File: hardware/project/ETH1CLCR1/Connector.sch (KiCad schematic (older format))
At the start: 25 parts, among them J1601 C64AC, K1601 HE3621A0510, K1602 HE3621A0510, K1603 HE3621A0510, K1604 HE3621A0510, K1605 HE3621A0510, K1606 HE3621A0510, Q1601 BC847W, Q1602 BC847W, Q1603 BC847W, Q1604 BC847W, Q1605 BC847W, Q1606 BC847W

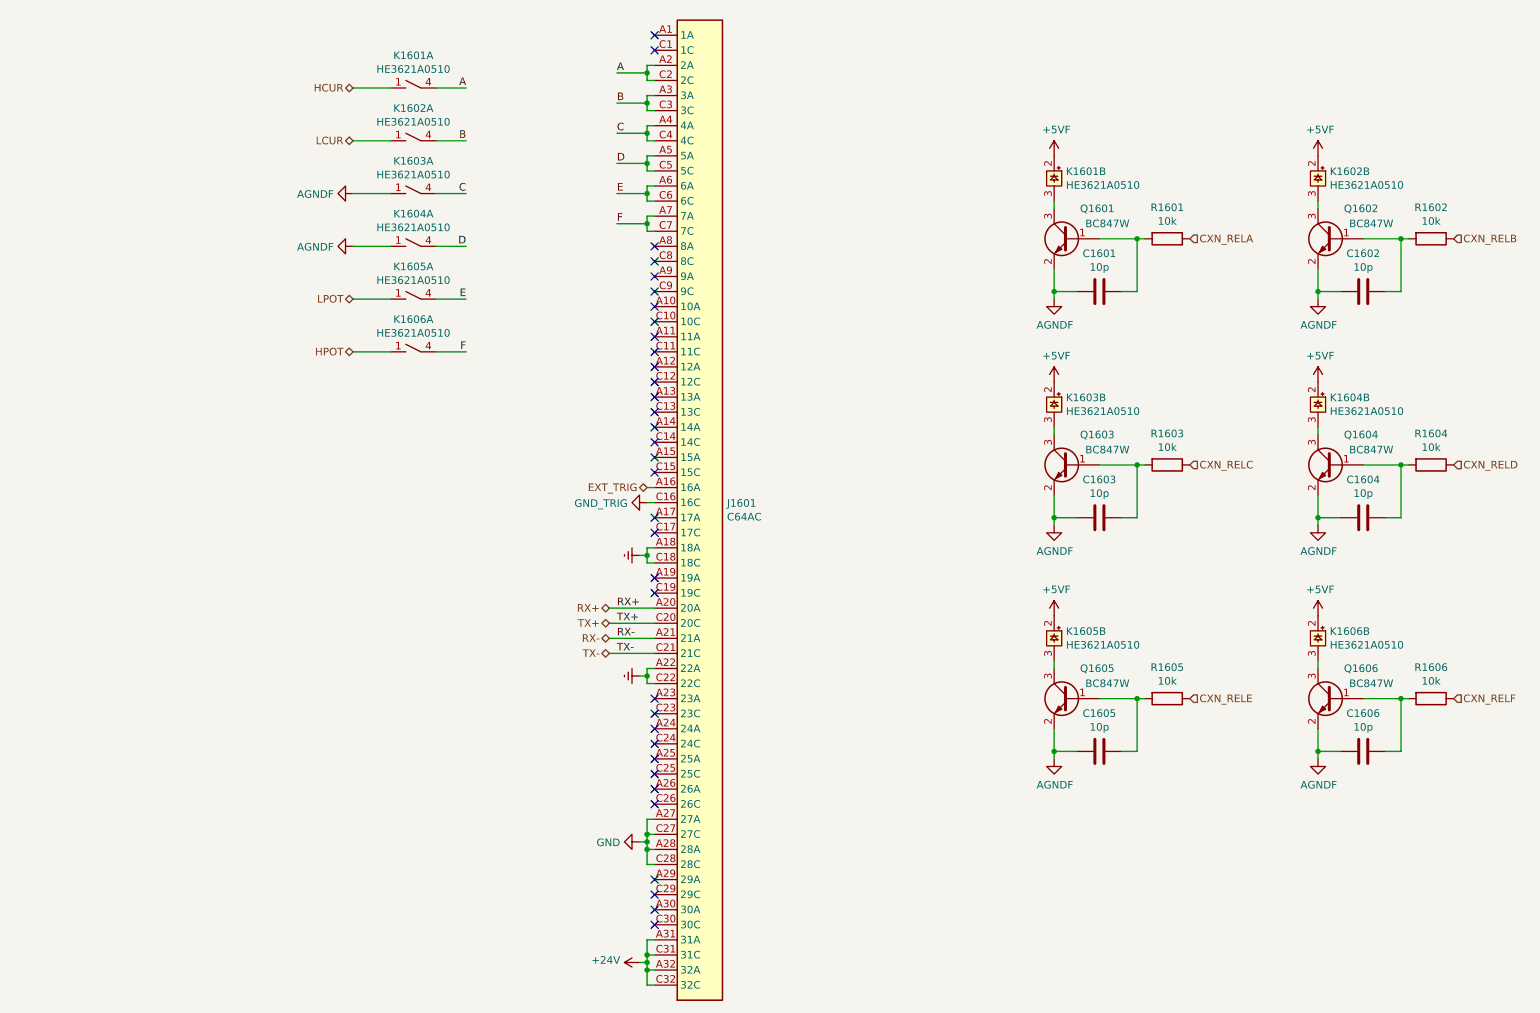
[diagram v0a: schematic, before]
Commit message: Modification in schematic and PCB layout.
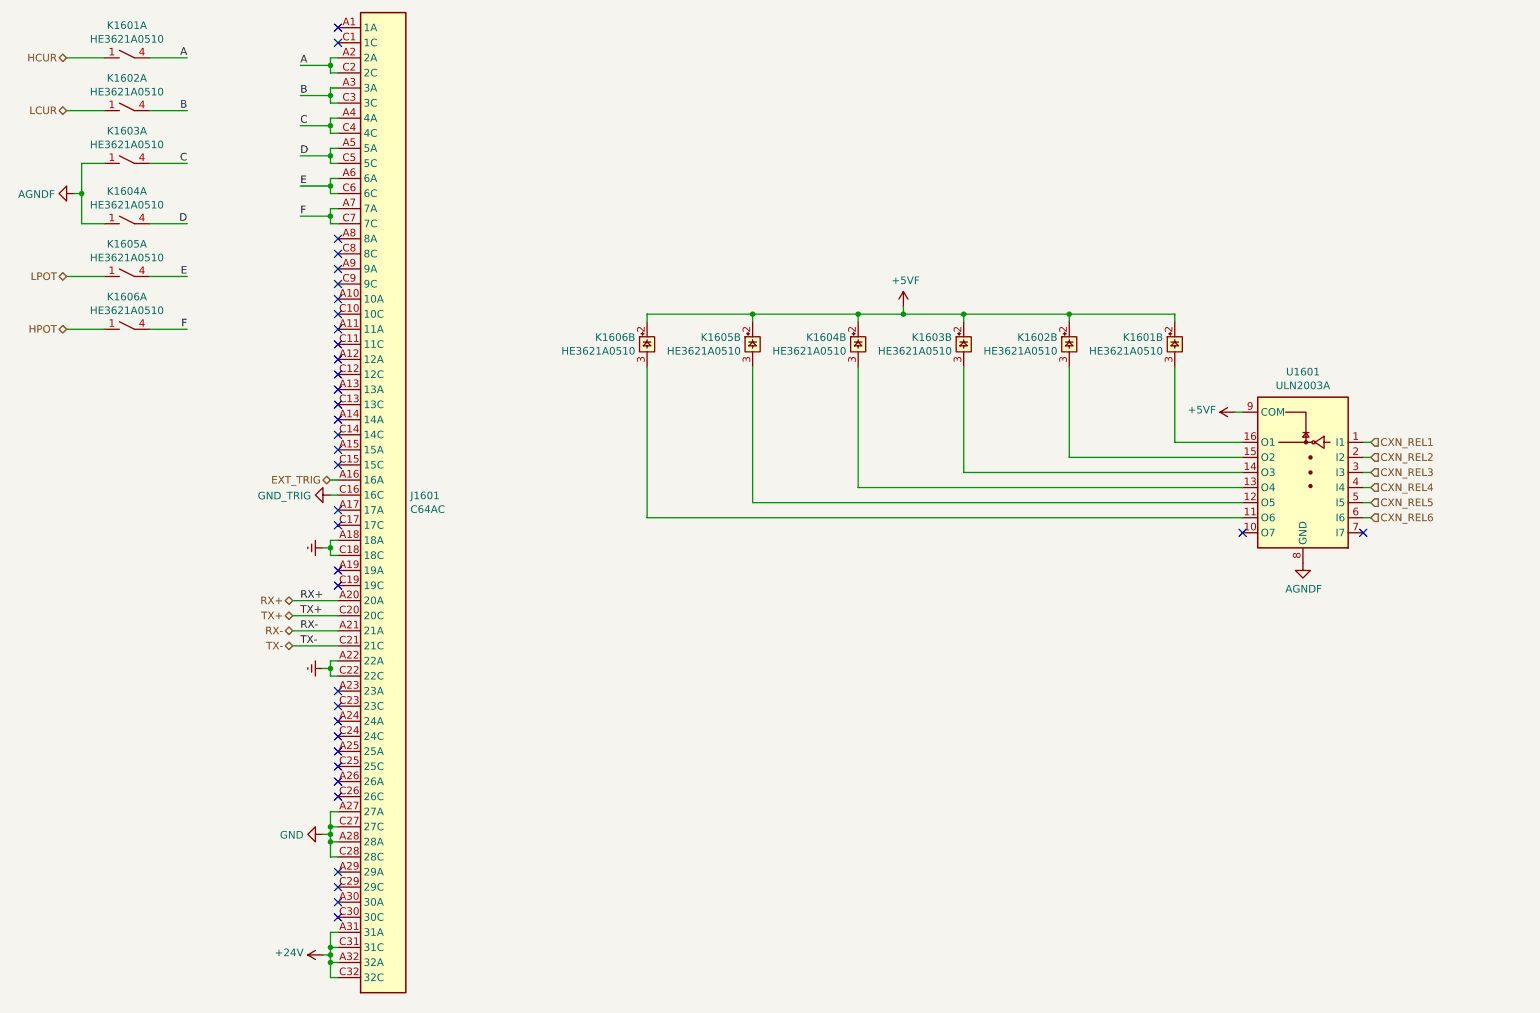
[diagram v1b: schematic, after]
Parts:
- removed C1601, C1602, C1603, C1604, C1605, C1606: 10p, Capacitor_SMD:C_0603_1608Metric_Pad1.05x0.95mm_HandSolder, symbol Device:C
- removed Q1601, Q1602, Q1603, Q1604, Q1605, Q1606: BC847W, Package_TO_SOT_SMD:SOT-323_SC-70, symbol Transistor_BJT:BC847W
- removed R1601, R1602, R1603, R1604, R1605, R1606: 10k, Resistor_SMD:R_0603_1608Metric_Pad1.05x0.95mm_HandSolder, symbol Device:R
- added U1601: ULN2003A, Package_SO:TSSOP-16_4.4x5mm_P0.65mm, symbol Transistor_Array:ULN2003A
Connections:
- net +5VF: now also U1601.9 (COM)
- net AGNDF: now also U1601.8 (GND)
- net at K1601.3: now also U1601.16 (O1)
- net at K1602.3: now also U1601.15 (O2)
- net at K1603.3: now also U1601.14 (O3)
- net at K1604.3: now also U1601.13 (O4)
- net at K1605.3: now also U1601.12 (O5)
- net at K1606.3: now also U1601.11 (O6)
- new net CXN_REL1: U1601.1 (I1)
- new net CXN_REL2: U1601.2 (I2)
- new net CXN_REL3: U1601.3 (I3)
- new net CXN_REL4: U1601.4 (I4)
- new net CXN_REL5: U1601.5 (I5)
- new net CXN_REL6: U1601.6 (I6)
- no-connect marks 34 -> 36
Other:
- moved on the sheet: J1601
